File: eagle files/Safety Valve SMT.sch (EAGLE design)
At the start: 31 parts, among them IC1 TL072

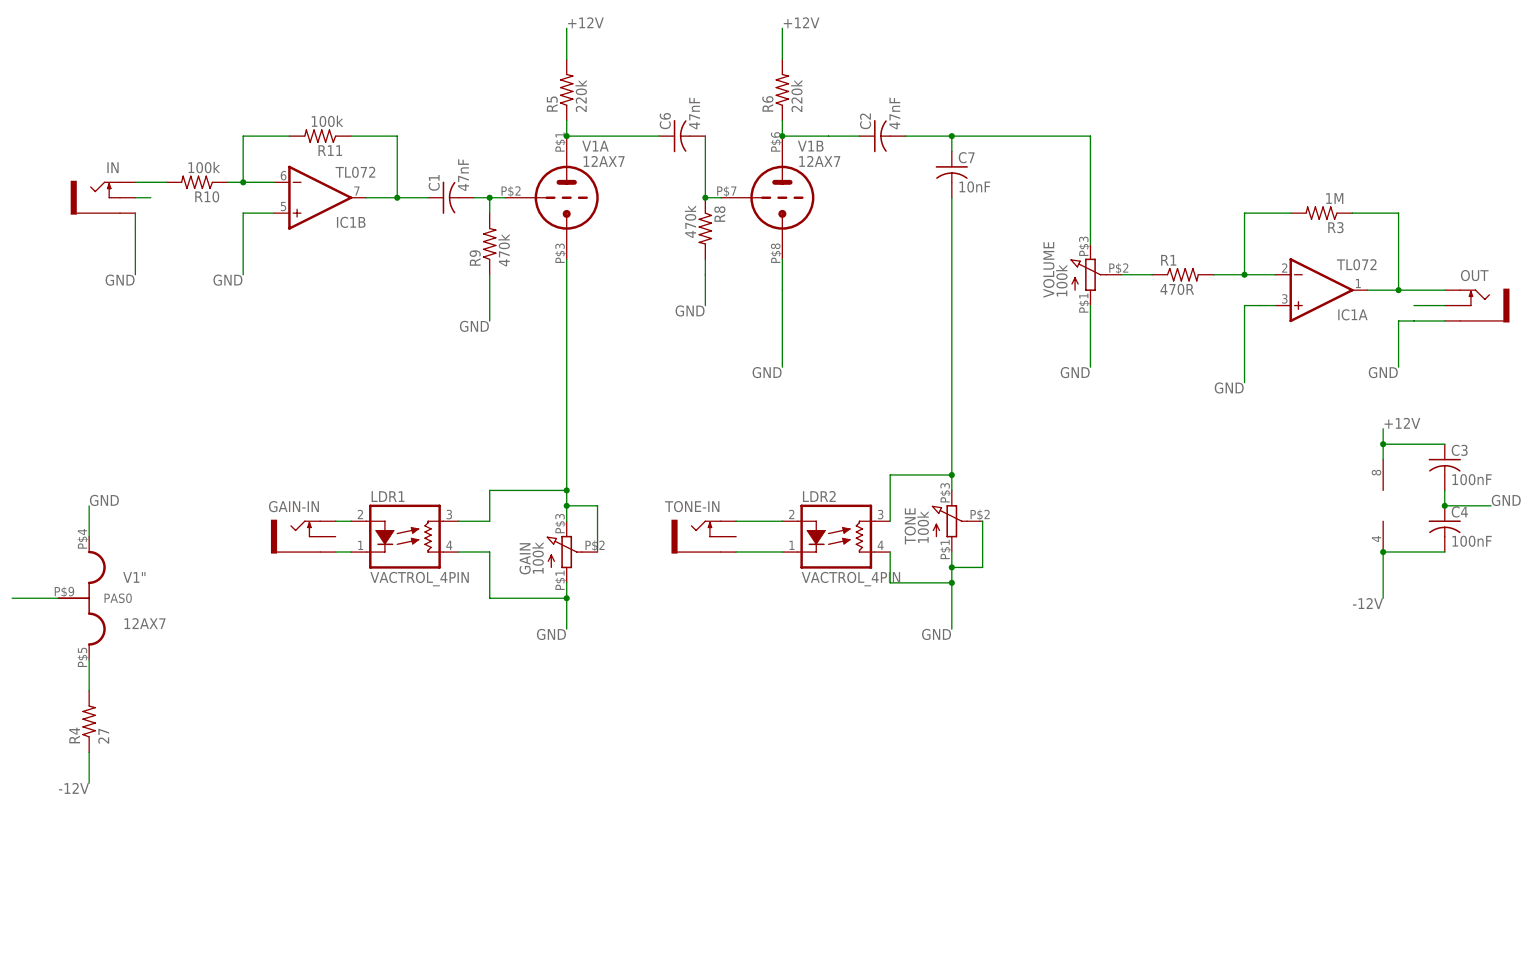
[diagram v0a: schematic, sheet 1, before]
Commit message: Added CV IN
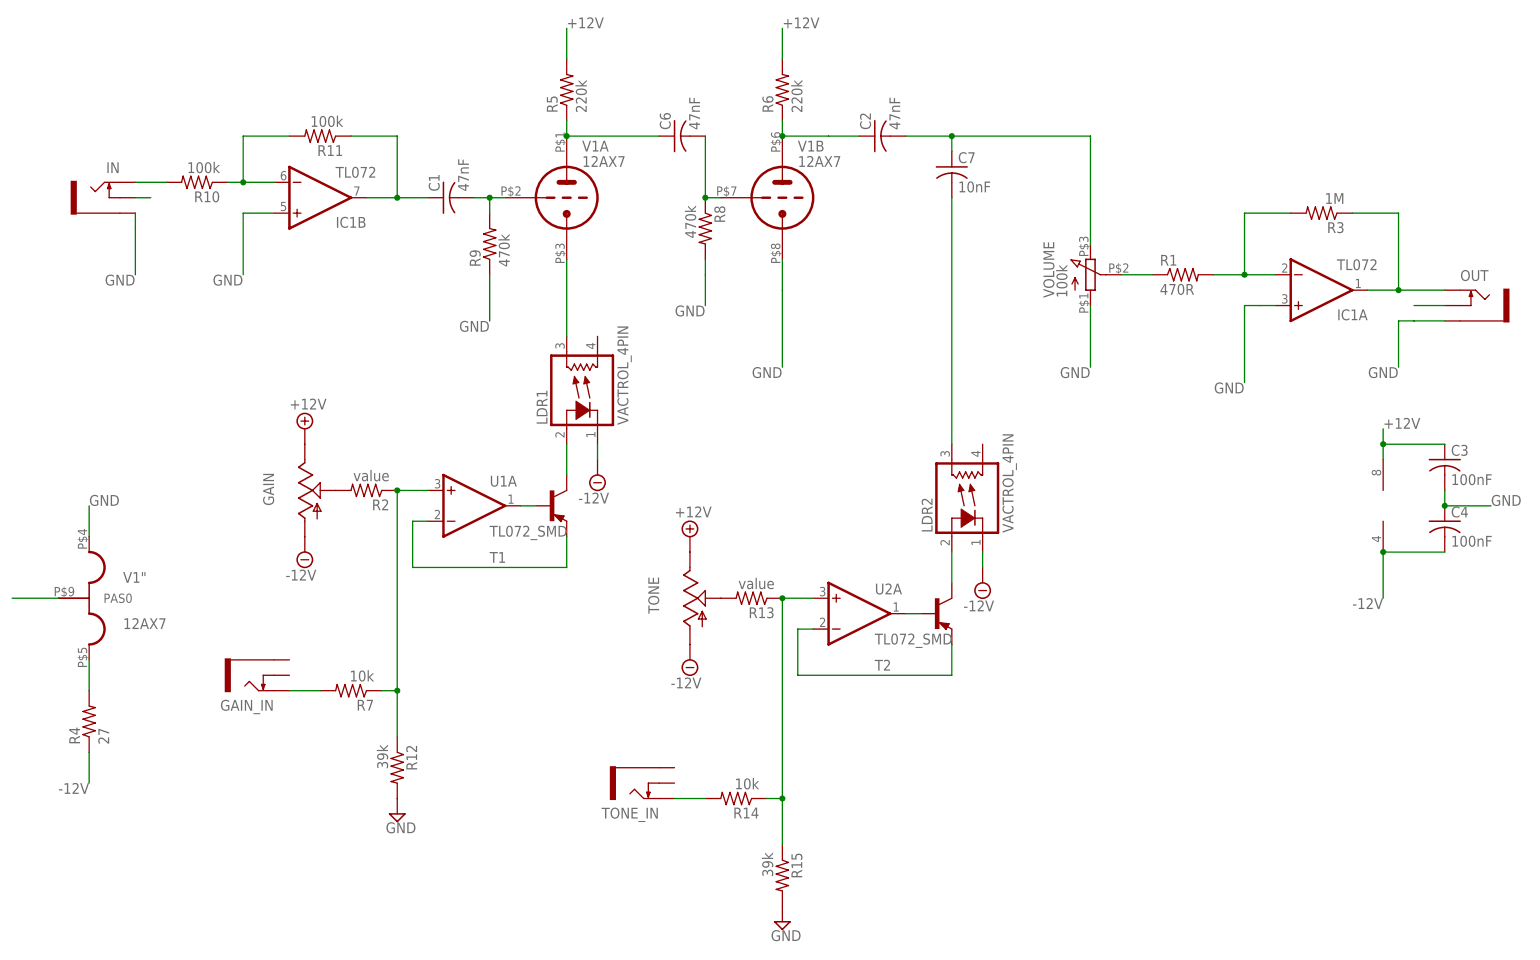
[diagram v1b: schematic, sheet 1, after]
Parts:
- removed GAIN-IN, TONE-IN: SOCKET_MONO_3.5MMPJ301M-12, GMSN:SOCKET_MONO_3.5MMPJ301M-12
- added GAIN_IN, TONE_IN: THONKICONNNEW, MusicThingModular:THONKICONNNEW
- added R12, R15: 39k, GMSN:RESISTOR_USR0805
- added R13, R2: value, GMSN:RESISTOR_USR0805
- added R14, R7: 10k, GMSN:RESISTOR_USR0805
- added T1, T2: (no value), MusicThingModular:BC807-16-PNP-SOT23-BEC
- added U1, U2: TL072_SMD, MusicThingModular:TL072_SMD
- GAIN, TONE: value 100k -> (none); device GMSN:RESISTOR_VARIABLE9MM_POT -> MusicThingModular:9MM_SNAP-IN_POT_; SPICEPREFIX X -> (none)
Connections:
- new net N$24: R12.1, R2.1, R7.1, U1A.+IN
- new net N$25: GAIN.S, R2.2
- new net N$26: GAIN_IN.TIP, R7.2
- new net N$27: LDR1.LED+, T1.C
- new net N$28: R13.1, R14.1, R15.1, U2A.+IN
- new net N$29: R13.2, TONE.S
- new net N$30: R14.2, TONE_IN.TIP
- new net N$31: LDR2.LED+, T2.C
- net +12V: now also GAIN.E, TONE.E
- net -12V: now also GAIN.A, LDR1.LED-, LDR2.LED-, TONE.A
- net GND: now also R12.2, R15.2; no longer GAIN.1, LDR1.RES2, LDR2.RES2, TONE.1, TONE.2
- net N$1: now also T2.E, U2A.-IN; no longer GAIN.2, GAIN.3, LDR1.RES1, V1A.TK
- net N$17: now also T2.B, U2A.OUT; no longer C7.2, LDR2.RES1, TONE.3
- net N$20: now also LDR1.RES1, V1A.TK; no longer LDR2.LED+, TONE-IN.TIP
- net N$21: now also C7.2, LDR2.RES1; no longer LDR2.LED-, TONE-IN.SLEEVE
- net N$22: now also T1.E, U1A.-IN; no longer GAIN-IN.TIP, LDR1.LED+
- net N$23: now also T1.B, U1A.OUT; no longer GAIN-IN.SLEEVE, LDR1.LED-
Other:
- moved on the sheet: LDR1, LDR2
